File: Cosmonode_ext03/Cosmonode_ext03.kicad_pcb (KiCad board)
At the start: 2 copper layers, 6 parts, among them J1 CONN_01X04, J2 GS3, J3 GS3, J4 CONN_01X04, J5 CONN_01X08, J6 CONN_01X08

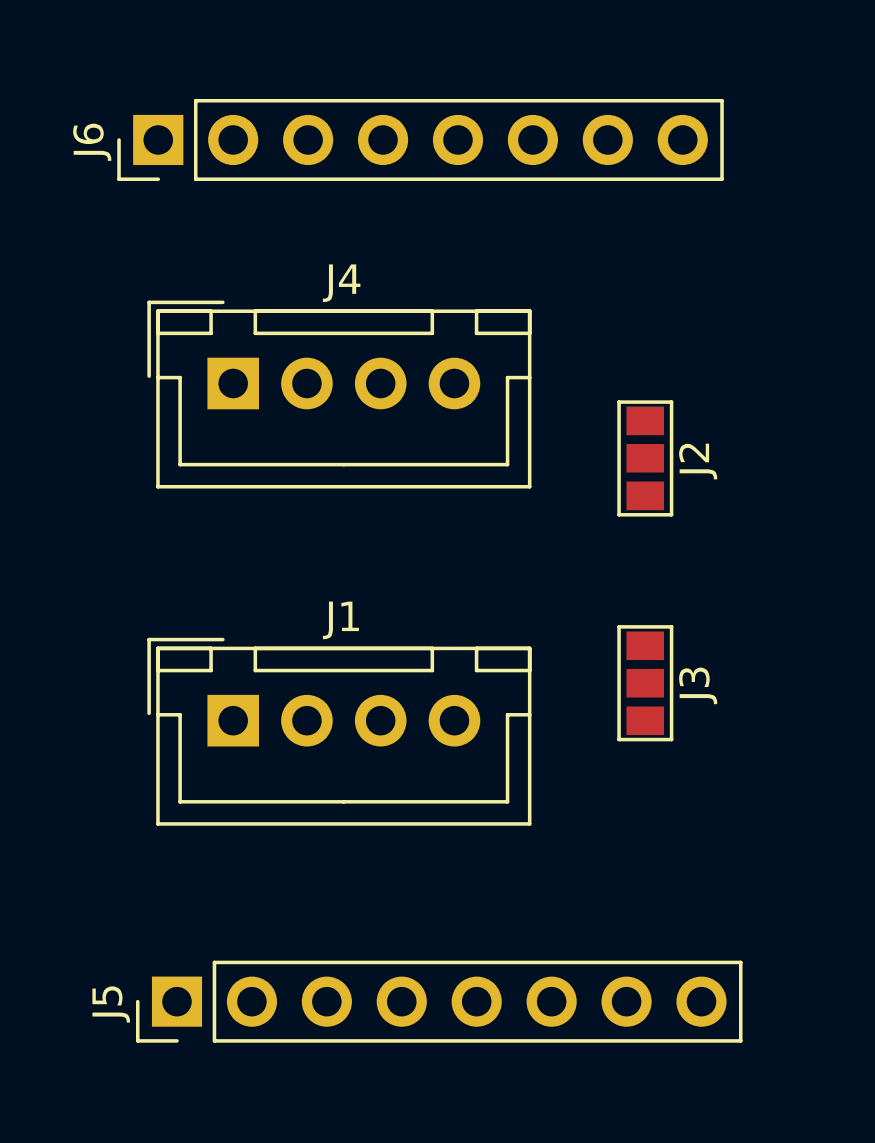
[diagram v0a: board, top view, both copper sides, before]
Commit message: big push!
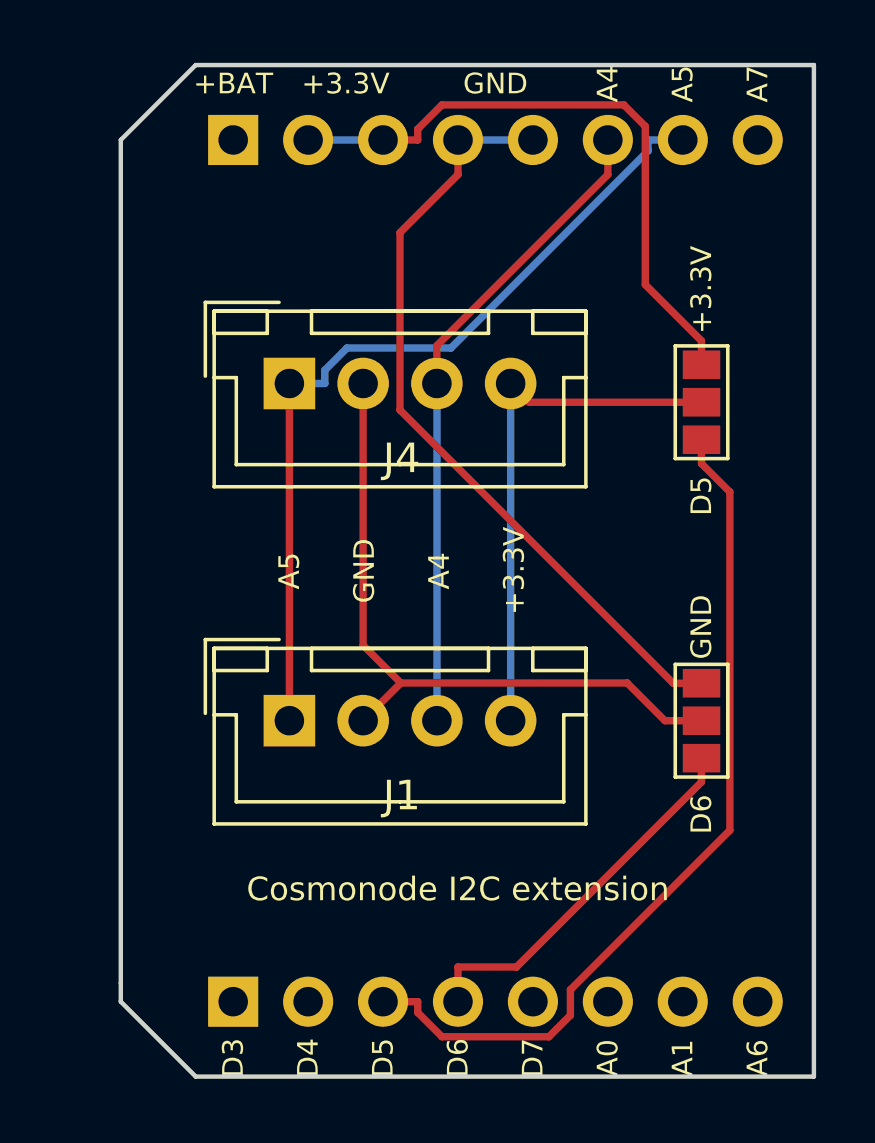
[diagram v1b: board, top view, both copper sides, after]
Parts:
- J5, J6: moved to B.Cu
- moved J2 2.69 mm to (166.4, 106.0)
- moved J6 2.54 mm to (150.5, 97.2), turned to 270 degrees
- moved J3 2.29 mm to (166.4, 116.8)
- moved J1 1.91 mm to (152.4, 116.8)
- moved J4 1.91 mm to (152.4, 105.4)
- moved J5 1.91 mm to (150.5, 126.4), turned to 270 degrees
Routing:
- net /D5: track 0.00 -> 29.5 mm
- net /A5: track 0.00 -> 28.7 mm
- net GND: track 0.00 -> 26.6 mm
- net Net-(J1-Pad2): track 0.00 -> 23.2 mm
- net /A4: track 0.00 -> 22.1 mm
- net +3V3: track 0.00 -> 21.3 mm
- net Net-(J1-Pad4): track 0.00 -> 18.2 mm
- net /D6: track 0.00 -> 12.8 mm
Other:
- board outline added: 23.5 x 34.3 mm
- board text added: "+3.3V"
- board text added: "+BAT"
- board text added: "A0"
- board text added: "A1"
- board text added: "A4"
- board text added: "A5"
- board text added: "A6"
- board text added: "A7"
- board text added: "Cosmonode I2C extension"
- board text added: "D3"
- board text added: "D4"
- board text added: "D5"
- board text added: "D6"
- board text added: "D7"
- board text added: "GND"
